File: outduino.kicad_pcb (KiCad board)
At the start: 2 copper layers, 44 x 86.5 mm, 123 parts, among them J1 USB_C_Receptacle_USB2.0, J2 Lichtenprog_conn, J3 USB_HDR, J4 QWIIC, J5 Conn_01x04, J6 I2C_HDR, J7 Conn_01x04, J8 Conn_01x04, J9 Conn_01x04, Q1 MMBT2222A, Q10 BC847, Q11 BC847, Q12 AO3401A, Q13 BC847, Q14 BC847, Q2 MMBT2222A, Q3 AO3401A, Q4 BC847, Q5 BC847, Q6 AO3401A, Q7 BC847, Q8 BC847, Q9 AO3401A, SW1 RST, SW3 B1/BOOT, SW4 B2, SW5 B2, U2 AZ1117-3.3, U3 ESP32-S3-WROOM-2

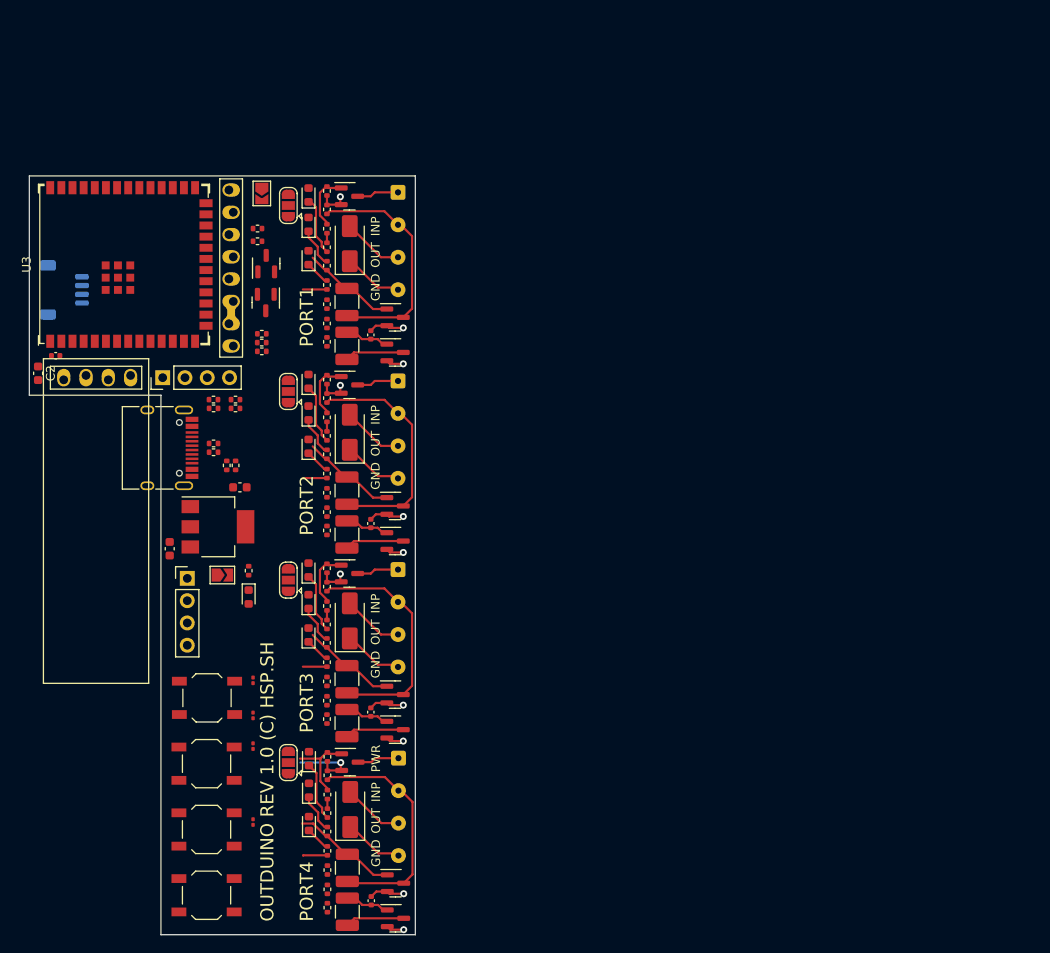
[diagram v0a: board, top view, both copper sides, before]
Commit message: before scripts
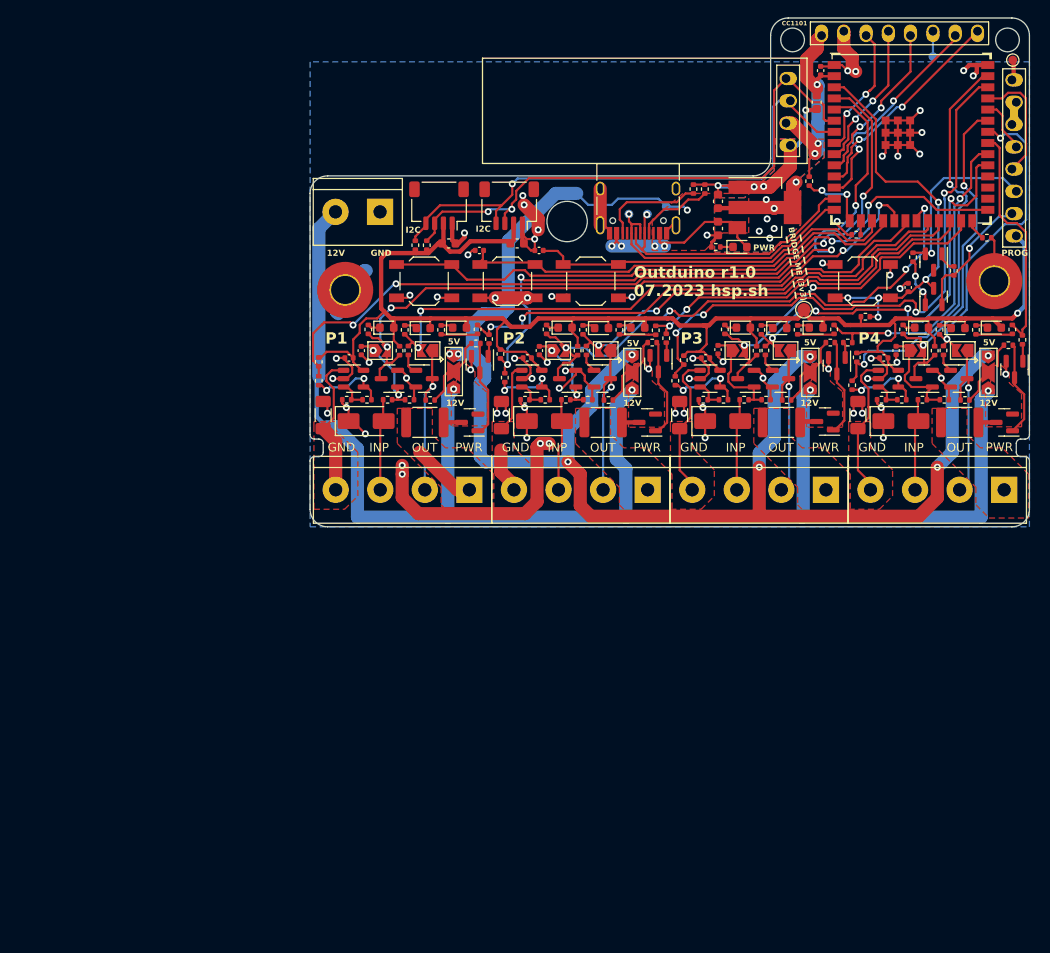
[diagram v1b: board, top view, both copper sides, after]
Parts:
- removed JP1: 3V3_FROM_USBC, Jumper:SolderJumper-2_P1.3mm_Open_TrianglePad1.0x1.5mm
- removed JP2: PWR_FROM_USBC, Jumper:SolderJumper-2_P1.3mm_Open_TrianglePad1.0x1.5mm
- added C10: 100n, Capacitor_SMD:C_0402_1005Metric, F.Cu at (82.4, 80.8)
- added C13: 100n, Capacitor_SMD:C_0402_1005Metric, F.Cu at (102.8, 80.8)
- added C14: 100n, Capacitor_SMD:C_0402_1005Metric, F.Cu at (123.1, 80.8)
- added C15: 100n, Capacitor_SMD:C_0402_1005Metric, F.Cu at (143.4, 80.8)
- added C16: 10u, Capacitor_SMD:C_0603_1608Metric, F.Cu at (101.6, 67.7)
- added C17: 10u, Capacitor_SMD:C_0603_1608Metric, F.Cu at (93.8, 67.7)
- added F1: 1812_2A, Fuse:Fuse_1812_4532Metric, F.Cu at (91.1, 88.1)
- added F2: 1812_2A, Fuse:Fuse_1812_4532Metric, F.Cu at (111.4, 88.1)
- added F3: 1812_2A, Fuse:Fuse_1812_4532Metric, F.Cu at (131.7, 88.1)
- added F4: 1812_2A, Fuse:Fuse_1812_4532Metric, F.Cu at (152.1, 88.1)
- added H1: SCR, MountingHole:MountingHole_3.2mm_M3_Pad_TopOnly, F.Cu at (82.0, 73.0)
- added H3: SCR, MountingHole:MountingHole_3.2mm_M3_Pad_TopOnly, F.Cu at (156.0, 72.0)
- added J10: CC1101_CONN, Critbit_lib:8pin_skewed, F.Cu at (145.2, 43.8)
- added JP10: OUT_BYP, Jumper:SolderJumper-2_P1.3mm_Open_TrianglePad1.0x1.5mm, F.Cu at (152.4, 79.9)
- added JP11: IN_BYP, Jumper:SolderJumper-2_P1.3mm_Open_TrianglePad1.0x1.5mm, F.Cu at (86.0, 79.9)
- added JP12: IN_BYP, Jumper:SolderJumper-2_P1.3mm_Open_TrianglePad1.0x1.5mm, F.Cu at (106.3, 79.9)
- added JP13: IN_BYP, Jumper:SolderJumper-2_P1.3mm_Open_TrianglePad1.0x1.5mm, F.Cu at (126.7, 79.9)
- added JP14: IN_BYP, Jumper:SolderJumper-2_P1.3mm_Open_TrianglePad1.0x1.5mm, F.Cu at (147.0, 79.9)
- added JP7: OUT_BYP, Jumper:SolderJumper-2_P1.3mm_Open_TrianglePad1.0x1.5mm, F.Cu at (91.4, 79.9)
- added JP8: OUT_BYP, Jumper:SolderJumper-2_P1.3mm_Open_TrianglePad1.0x1.5mm, F.Cu at (111.7, 79.9)
- added JP9: OUT_BYP, Jumper:SolderJumper-2_P1.3mm_Open_TrianglePad1.0x1.5mm, F.Cu at (132.2, 79.9)
- added Q15: BC847, Package_TO_SOT_SMD:SOT-23, F.Cu at (97.3, 81.5)
- added Q16: BC847, Package_TO_SOT_SMD:SOT-23, F.Cu at (117.7, 81.4)
- added Q17: BC847, Package_TO_SOT_SMD:SOT-23, F.Cu at (138.1, 81.6)
- added Q18: BC847, Package_TO_SOT_SMD:SOT-23, F.Cu at (158.3, 82.1)
- added R17: 50mR/1206, Resistor_SMD:R_1206_3216Metric_Pad1.30x1.75mm_HandSolder, F.Cu at (99.8, 87.3)
- added R37: 330/0.1%, Resistor_SMD:R_0402_1005Metric, F.Cu at (102.5, 85.5)
- added R49: 10k, Resistor_SMD:R_0402_1005Metric, F.Cu at (84.5, 85.5)
- added R61: 10k, Resistor_SMD:R_0402_1005Metric, F.Cu at (145.4, 85.5)
- added R64: 1k, Resistor_SMD:R_0402_1005Metric, F.Cu at (79.0, 83.3)
- added R65: 1k, Resistor_SMD:R_0402_1005Metric, F.Cu at (100.2, 83.0)
- added R66: 1k, Resistor_SMD:R_0402_1005Metric, F.Cu at (119.6, 83.3)
- added R67: 1k, Resistor_SMD:R_0402_1005Metric, F.Cu at (139.8, 83.9)
- added R68: 10k, Resistor_SMD:R_0402_1005Metric, F.Cu at (79.0, 81.2)
- added R69: 10k, Resistor_SMD:R_0402_1005Metric, F.Cu at (99.7, 80.3)
- added R70: 10k, Resistor_SMD:R_0402_1005Metric, F.Cu at (120.6, 81.0)
- added R71: 10k, Resistor_SMD:R_0402_1005Metric, F.Cu at (140.3, 80.7)
- added R72: 10k, Resistor_SMD:R_0402_1005Metric, F.Cu at (98.4, 78.6)
- added R73: 10k, Resistor_SMD:R_0402_1005Metric, F.Cu at (118.6, 78.5)
- added R74: 10k, Resistor_SMD:R_0402_1005Metric, F.Cu at (139.3, 79.0)
- added R75: 10k, Resistor_SMD:R_0402_1005Metric, F.Cu at (159.2, 78.7)
- added TP1: IOPAD, TestPoint:TestPoint_Pad_D1.0mm, B.Cu at (118.6, 63.5)
- added TP2: IOPAD, TestPoint:TestPoint_Pad_D1.0mm, B.Cu at (114.3, 64.3)
- added TP3: IOPAD, TestPoint:TestPoint_Pad_D1.0mm, B.Cu at (116.5, 64.3)
- added TP4: IOPAD, TestPoint:TestPoint_Pad_D1.0mm, F.Cu at (158.1, 46.8)
- added TP5: IOPAD, TestPoint:TestPoint_Pad_D1.0mm, B.Cu at (149.0, 46.4)
- added TP6: IOPAD, TestPoint:TestPoint_Pad_D1.5mm, F.Cu at (134.3, 75.2)
- added U4: LMV321, Package_TO_SOT_SMD:SOT-23-5, F.Cu at (83.0, 83.1)
- added U5: LMV321, Package_TO_SOT_SMD:SOT-23-5, F.Cu at (103.3, 83.1)
- added U6: LMV321, Package_TO_SOT_SMD:SOT-23-5, F.Cu at (123.6, 83.1)
- added U7: LMV321, Package_TO_SOT_SMD:SOT-23-5, F.Cu at (143.9, 83.1)
- C11, C12, C8: footprint Capacitor_SMD:C_0201_0603Metric -> Capacitor_SMD:C_0402_1005Metric
- J3: value USB_HDR -> Conn_01x02; footprint Connector_PinHeader_2.54mm:PinHeader_1x04_P2.54mm_Vertical -> TerminalBlock:TerminalBlock_bornier-2_P5.08mm
- J4: moved to F.Cu
- J5, J7, J8, J9: footprint Connector_Wire:SolderWire-0.127sqmm_1x04_P3.7mm_D0.48mm_OD1mm -> TerminalBlock:TerminalBlock_bornier-4_P5.08mm
- J6: value I2C_HDR -> QWIIC; footprint Connector_PinHeader_2.54mm:PinHeader_1x04_P2.54mm_Vertical -> Connector_JST:JST_SH_SM04B-SRSS-TB_1x04-1MP_P1.00mm_Horizontal
- JP3, JP4, JP5, JP6: footprint Jumper:SolderJumper-3_P1.3mm_Open_RoundedPad1.0x1.5mm -> Jumper:SolderJumper-3_P2.0mm_Open_TrianglePad1.0x1.5mm
- R10, R11, R12, R9: value 22R/0603 -> 10k
- R13: value 33k -> 10k
- R20, R34, R6: value DNP/1210 -> 50mR/1206; footprint Resistor_SMD:R_1210_3225Metric_Pad1.30x2.65mm_HandSolder -> Resistor_SMD:R_1206_3216Metric_Pad1.30x1.75mm_HandSolder
- R25: footprint Resistor_SMD:R_0201_0603Metric -> Resistor_SMD:R_0402_1005Metric
- R36, R46, R48: value DNP/1210 -> 330/0.1%; footprint Resistor_SMD:R_1210_3225Metric_Pad1.30x2.65mm_HandSolder -> Resistor_SMD:R_0402_1005Metric
- R58, R60: value DNP/1210 -> 10k; footprint Resistor_SMD:R_1210_3225Metric_Pad1.30x2.65mm_HandSolder -> Resistor_SMD:R_0402_1005Metric
- moved R55 94.4 mm to (158.1, 77.5)
- moved C2 94.0 mm to (135.8, 51.6)
- moved R59 93.9 mm to (149.2, 79.9)
- moved C1 93.1 mm to (136.2, 48.0), turned to 90 degrees
- moved D17 92.3 mm to (156.0, 77.3), turned to 0 degrees
- moved R52 92.2 mm to (153.9, 77.5), turned to 90 degrees
- moved JP6 91.3 mm to (155.3, 82.4), turned to -90 degrees
- moved U3 91.0 mm to (146.5, 55.6), turned to 0 degrees
- moved D18 90.8 mm to (151.9, 77.3), turned to 0 degrees
- moved R57 90.7 mm to (157.6, 79.3), turned to 180 degrees
- moved R53 90.2 mm to (149.8, 77.5)
- moved J2 90.1 mm to (158.2, 58.0), turned to 180 degrees
- moved D19 89.8 mm to (147.7, 77.3), turned to 0 degrees
- moved R63 89.8 mm to (150.3, 85.5), turned to 180 degrees
- moved C8 89.2 mm to (146.2, 72.7), turned to 90 degrees
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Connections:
- net /ESP_BOOT renamed /ESP_BOOT_B1
- net Net-(D11-A2) renamed /IO_block2/INP_BANK
- net Net-(D16-A2) renamed /IO_block3/INP_BANK
- net Net-(D21-A2) renamed /IO_block4/INP_BANK
- net Net-(D3-A2) renamed /IO_block1/INP_BANK
- C5 pad 1: Net-(Q5-B) -> Net-(JP11-A)
- C6 pad 1: Net-(Q8-B) -> Net-(JP12-A)
- C7 pad 1: Net-(Q11-B) -> Net-(JP13-A)
- C9 pad 1: Net-(Q14-B) -> Net-(JP14-A)
- J1 pad A6: Net-(J1-D+-PadA6) -> /USBDP
- J1 pad A7: Net-(J1-D--PadA7) -> /USBDM
- J1 pad B6: Net-(J1-D+-PadA6) -> /USBDP
- J1 pad B7: Net-(J1-D--PadA7) -> /USBDM
- J2 pad 1: Net-(J2-VDD) -> +3.3V
- J3 pad 1: VBUS -> GND
- J3 pad 2: Net-(J3-Pin_2) -> +12V
- J5 pad 1: Net-(J5-Pin_1) -> /IO_block1/PWR_BANK
- J5 pad 2: Net-(J5-Pin_2) -> /IO_block1/OUT_BANK
- J5 pad 4: GND -> /IO_block1/GND_BANK
- J7 pad 1: Net-(J7-Pin_1) -> /IO_block2/PWR_BANK
- J7 pad 2: Net-(J7-Pin_2) -> /IO_block2/OUT_BANK
- J7 pad 4: GND -> /IO_block2/GND_BANK
- J8 pad 1: Net-(J8-Pin_1) -> /IO_block3/PWR_BANK
- J8 pad 2: Net-(J8-Pin_2) -> /IO_block3/OUT_BANK
- J8 pad 4: GND -> /IO_block3/GND_BANK
- J9 pad 1: Net-(J9-Pin_1) -> /IO_block4/PWR_BANK
- J9 pad 2: Net-(J9-Pin_2) -> /IO_block4/OUT_BANK
- J9 pad 4: GND -> /IO_block4/GND_BANK
- Q10 pad 1: /OUT3 -> Net-(Q10-B)
- Q10 pad 3: Net-(J8-Pin_2) -> /IO_block3/OUT_BANK
- Q11 pad 1: Net-(Q11-B) -> Net-(JP13-A)
- Q12 pad 1: /PWR4 -> Net-(Q12-G)
- Q12 pad 3: Net-(J9-Pin_1) -> Net-(Q12-D)
- Q13 pad 1: /OUT4 -> Net-(Q13-B)
- Q13 pad 3: Net-(J9-Pin_2) -> /IO_block4/OUT_BANK
- Q14 pad 1: Net-(Q14-B) -> Net-(JP14-A)
- Q3 pad 1: /PWR1 -> Net-(Q15-C)
- Q3 pad 3: Net-(J5-Pin_1) -> Net-(Q3-D)
- Q4 pad 1: /OUT1 -> Net-(Q4-B)
- Q4 pad 3: Net-(J5-Pin_2) -> /IO_block1/OUT_BANK
- Q5 pad 1: Net-(Q5-B) -> Net-(JP11-A)
- Q6 pad 1: /PWR2 -> Net-(Q16-C)
- Q6 pad 3: Net-(J7-Pin_1) -> Net-(Q6-D)
- Q7 pad 1: /OUT2 -> Net-(Q7-B)
- Q7 pad 3: Net-(J7-Pin_2) -> /IO_block2/OUT_BANK
- Q8 pad 1: Net-(Q8-B) -> Net-(JP12-A)
- Q9 pad 1: /PWR3 -> Net-(Q17-C)
- Q9 pad 3: Net-(J8-Pin_1) -> Net-(Q9-D)
- R10 pad 1: Net-(J1-D+-PadA6) -> Net-(Q7-B)
- R10 pad 2: /USBDP -> /OUT2
- R11 pad 1: Net-(J3-Pin_2) -> Net-(Q10-B)
- R11 pad 2: /USBDP -> /OUT3
- R12 pad 1: Net-(J3-Pin_3) -> Net-(Q13-B)
- R12 pad 2: /USBDM -> /OUT4
- R14 pad 1: /PWR1 -> Net-(Q15-C)
- R15 pad 1: Net-(J5-Pin_2) -> /IO_block1/OUT_BANK
- R18 pad 2: Net-(Q5-B) -> Net-(JP11-A)
- R19 pad 2: Net-(Q5-B) -> Net-(JP11-A)
- R20 pad 1: Net-(Q5-B) -> /IO_block3/GND_BANK
- R20 pad 2: /IN1 -> GND
- R30 pad 2: VDD -> +3.3V
- R32 pad 1: Net-(J7-Pin_2) -> /IO_block2/OUT_BANK
- R33 pad 1: /PWR2 -> Net-(Q16-C)
- R34 pad 1: /OUT2 -> /IO_block4/GND_BANK
- R34 pad 2: Net-(J7-Pin_2) -> GND
- R36 pad 1: Net-(Q8-B) -> Net-(U4--)
- R36 pad 2: /IN2 -> GND
- R38 pad 2: Net-(Q8-B) -> Net-(JP12-A)
- R39 pad 2: Net-(Q8-B) -> Net-(JP12-A)
- R44 pad 1: Net-(J8-Pin_2) -> /IO_block3/OUT_BANK
- R45 pad 1: /PWR3 -> Net-(Q17-C)
- R46 pad 1: /OUT3 -> Net-(U6--)
- R46 pad 2: Net-(J8-Pin_2) -> GND
- R48 pad 1: Net-(Q11-B) -> Net-(U7--)
- R48 pad 2: /IN3 -> GND
- R50 pad 2: Net-(Q11-B) -> Net-(JP13-A)
- R51 pad 2: Net-(Q11-B) -> Net-(JP13-A)
- R56 pad 1: Net-(J9-Pin_2) -> /IO_block4/OUT_BANK
- R57 pad 1: /PWR4 -> Net-(Q12-G)
- R58 pad 1: /OUT4 -> Net-(R58-Pad1)
- R58 pad 2: Net-(J9-Pin_2) -> Net-(U5--)
- R6 pad 1: /OUT1 -> /IO_block1/GND_BANK
- R6 pad 2: Net-(J5-Pin_2) -> GND
- R60 pad 1: Net-(Q14-B) -> Net-(R60-Pad1)
- R60 pad 2: /IN4 -> Net-(U6--)
- R62 pad 2: Net-(Q14-B) -> Net-(JP14-A)
- R63 pad 2: Net-(Q14-B) -> Net-(JP14-A)
- R9 pad 1: Net-(J1-D--PadA7) -> Net-(Q4-B)
- R9 pad 2: /USBDM -> /OUT1
- U3 pad 10: /OUT4 -> /CC1101_SO
- U3 pad 11: /IN4 -> /CC1101_CSn
- U3 pad 12: /OUT1 -> /CC1101_GDO0
- U3 pad 17: /IN1 -> /ESP_B2
- U3 pad 18: /PWR2 -> /ESP_B3
- U3 pad 19: /OUT2 -> /IN1
- U3 pad 20: /IN2 -> /OUT1
- U3 pad 21: /PWR3 -> /IN2
- U3 pad 22: /OUT3 -> /PWR1
- U3 pad 23: unconnected-(U3-GPIO21-Pad23) -> /OUT2
- U3 pad 24: unconnected-(U3-GPIO47/SPICLK_P/SUBSPICLK_P_DIFF-Pad24) -> /PWR2
- U3 pad 25: unconnected-(U3-GPIO48/SPICLK_N/SUBSPICLK_N_DIFF-Pad25) -> /IN3
- U3 pad 31: unconnected-(U3-GPIO38/FSPIWP/SUBSPIWP-Pad31) -> /OUT3
- U3 pad 32: /ESP_B2 -> /PWR3
- U3 pad 33: /ESP_B3 -> /PWR4
- U3 pad 34: unconnected-(U3-MTDI/GPIO41/CLK_OUT1-Pad34) -> /OUT4
- U3 pad 35: unconnected-(U3-MTMS/GPIO42-Pad35) -> /IN4
- U3 pad 36: /PROG_TX -> /TARG_RX
- U3 pad 37: /PROG_RX -> /TARG_TX
- U3 pad 38: unconnected-(U3-GPIO2/TOUCH2/ADC1_CH1-Pad38) -> /CURR3
- U3 pad 39: unconnected-(U3-GPIO1/TOUCH1/ADC1_CH0-Pad39) -> /CURR4
- U3 pad 4: unconnected-(U3-GPIO4/TOUCH4/ADC1_CH3-Pad4) -> /CURR2
- U3 pad 5: /SCL -> /CURR1
- U3 pad 7: /PWR1 -> /SCL
- U3 pad 8: /IN3 -> /CC1101_SI
- U3 pad 9: /PWR4 -> /CC1101_SCLK
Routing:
- net +3.3V: track 0.00 -> 224.4 mm, vias 0 -> 11
- net GND: track 51.6 -> 243.5 mm, vias 8 -> 70
- net VBUS: track 0.00 -> 191.2 mm, vias 0 -> 13
- net +12V: track 0.00 -> 169.1 mm, vias 0 -> 4
- net /CURR1: track 0.00 -> 92.8 mm, vias 0 -> 4
- net /ESP_BOOT_B1: track 0.00 -> 74.5 mm, vias 0 -> 2
- net /CURR2: track 0.00 -> 72.5 mm, vias 0 -> 4
- net /IN1: track 9.50 -> 78.0 mm, vias 0 -> 4
- net /CURR3: track 0.00 -> 67.3 mm, vias 0 -> 4
- net /SDA: track 0.00 -> 66.0 mm, vias 0 -> 2
- net /SCL: track 0.00 -> 63.9 mm, vias 0 -> 1
- net /OUT1: track 11.0 -> 68.3 mm, vias 0 -> 2
- net /IN2: track 9.50 -> 63.3 mm, vias 0 -> 4
- net /PWR1: track 6.50 -> 59.4 mm, vias 0 -> 2
- net /ESP_B3: track 0.00 -> 51.9 mm
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- added copper zone on B.Cu, net +3.3V
- added copper zone on F.Cu, net +3.3V
- added copper zone on F.Cu, net /IO_block1/GND_BANK
- added copper zone on F.Cu, net /IO_block1/PWR
- added copper zone on F.Cu, net /IO_block1/PWR_BANK
- added copper zone on F.Cu, net /IO_block2/GND_BANK
- added copper zone on F.Cu, net /IO_block2/PWR
- added copper zone on F.Cu, net /IO_block2/PWR_BANK
- added copper zone on F.Cu, net /IO_block3/GND_BANK
- added copper zone on F.Cu, net /IO_block3/PWR
- added copper zone on F.Cu, net /IO_block3/PWR_BANK
- added copper zone on F.Cu, net /IO_block4/GND_BANK
- added copper zone on F.Cu, net /IO_block4/PWR
- added copper zone on F.Cu, net /IO_block4/PWR_BANK
- added copper zone on B.Cu, net GND
- added copper zone on F.Cu, net VBUS
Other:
- board size 44 x 86.5 mm -> 82 x 58 mm
- board text added: "12V"
- board text added: "5V"
- board text added: "BRIDGE ME (3v3)"
- board text added: "CC1101"
- board text added: "DM"
- board text added: "DP"
- board text added: "I2C"
- board text added: "Outduino r1.0 07.2023 hsp.sh"
- board text added: "P1"
- board text added: "P2"
- board text added: "P3"
- board text added: "P4"
- board text added: "PROG"
- board text removed: "OUTDUINO REV 1.0 (C) HSP.SH"
- board text removed: "PORT1"
- board text removed: "PORT2"
- board text removed: "PORT3"
- board text removed: "PORT4"
